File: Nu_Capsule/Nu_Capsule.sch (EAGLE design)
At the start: 20 parts, among them T1 2SC3324, T2 2SC3324

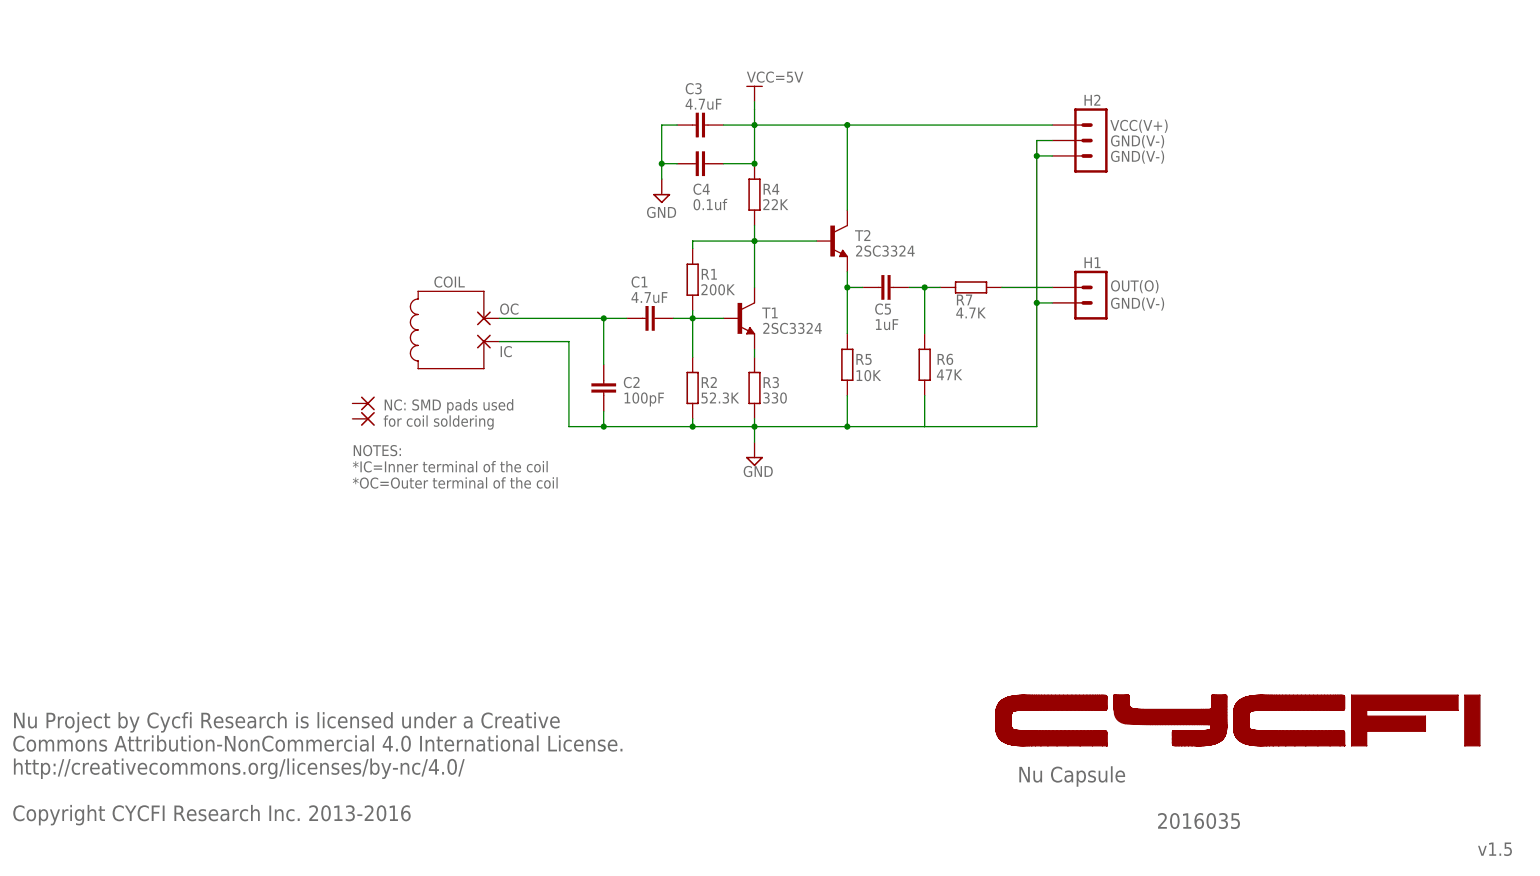
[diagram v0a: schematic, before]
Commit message: Doc updates
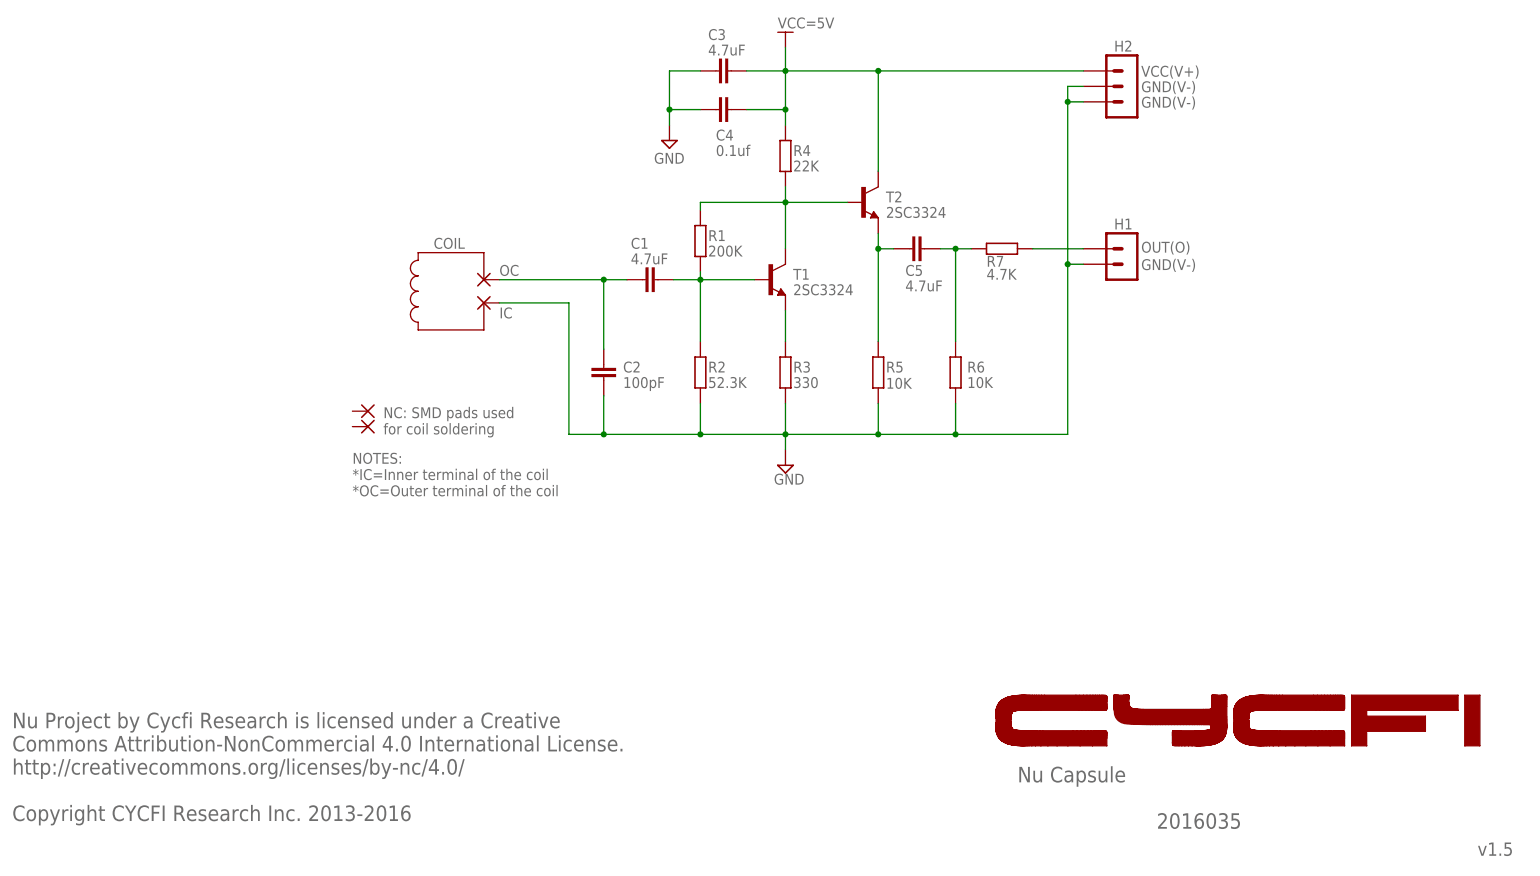
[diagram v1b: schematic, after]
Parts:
- C5: value 1uF -> 4.7uF
- R6: value 47K -> 10K
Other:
- moved on the sheet: C1, C2, C3, C4, C5, H1, H2, R1, R2, R3, R4, R5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

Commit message: updates and minor corrections
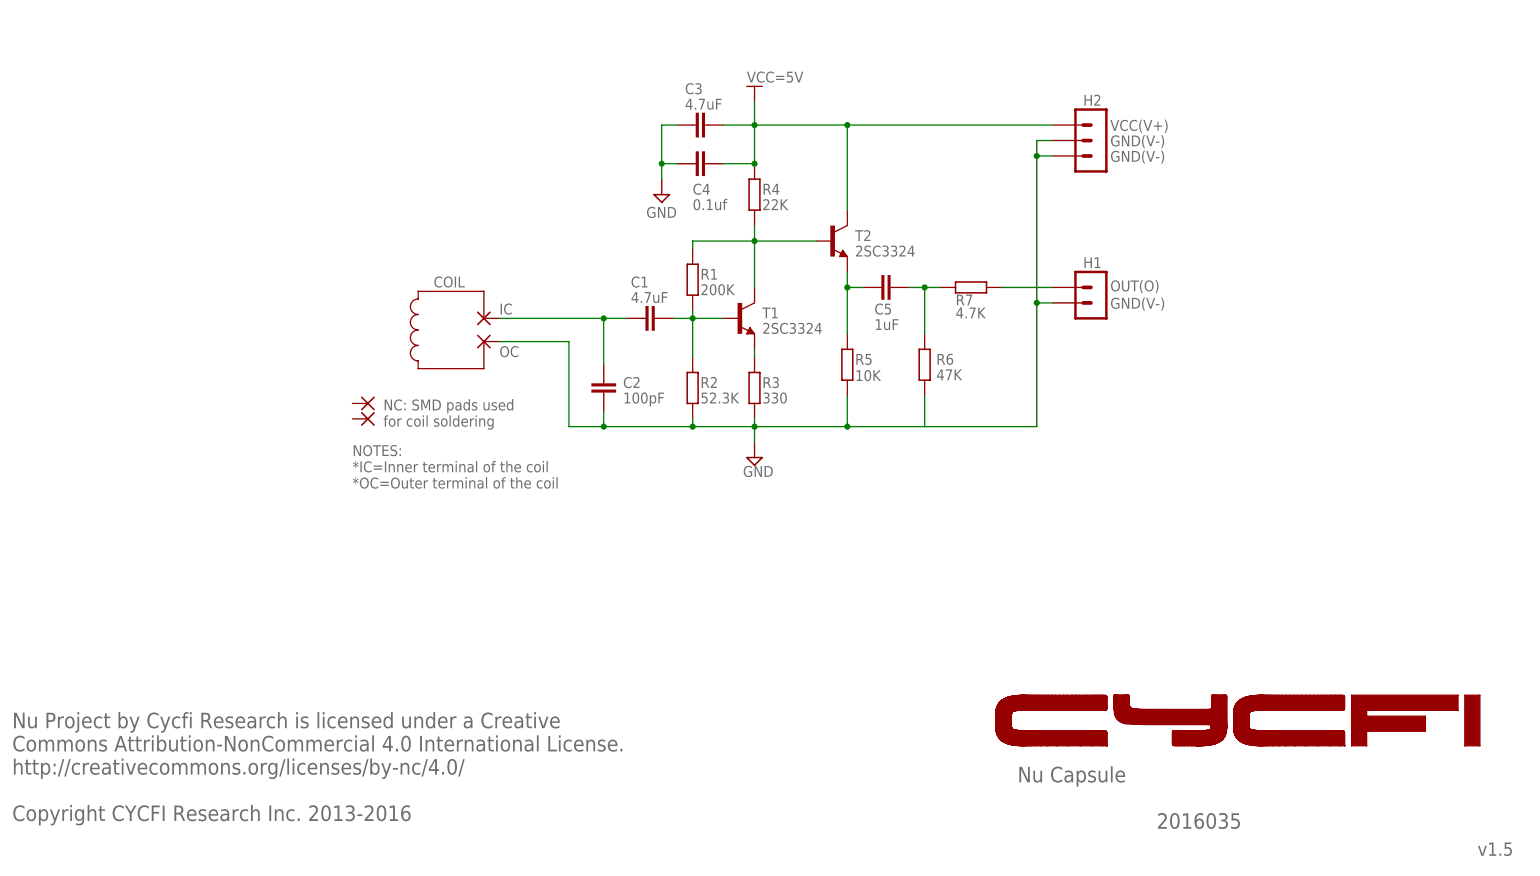
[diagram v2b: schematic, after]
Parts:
- C5: value 4.7uF -> 1uF
- R6: value 10K -> 47K
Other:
- moved on the sheet: C1, C2, C3, C4, C5, H1, H2, R1, R2, R3, R4, R5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

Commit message: more updates; tweaks
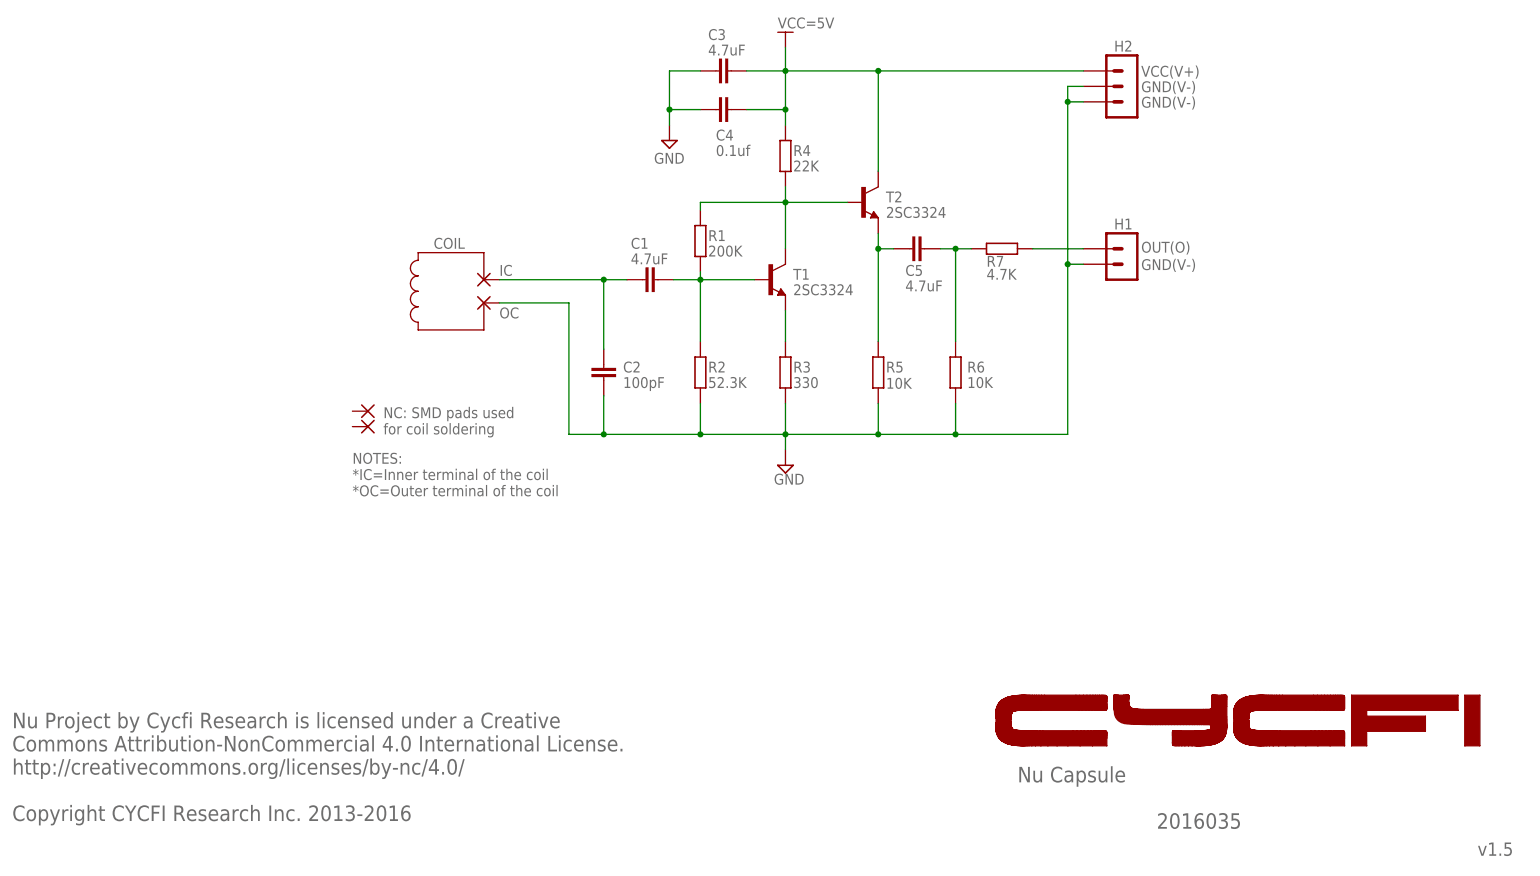
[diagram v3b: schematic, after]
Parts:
- C5: value 1uF -> 4.7uF
- R6: value 47K -> 10K
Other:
- moved on the sheet: C1, C2, C3, C4, C5, H1, H2, R1, R2, R3, R4, R5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

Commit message: Licenses
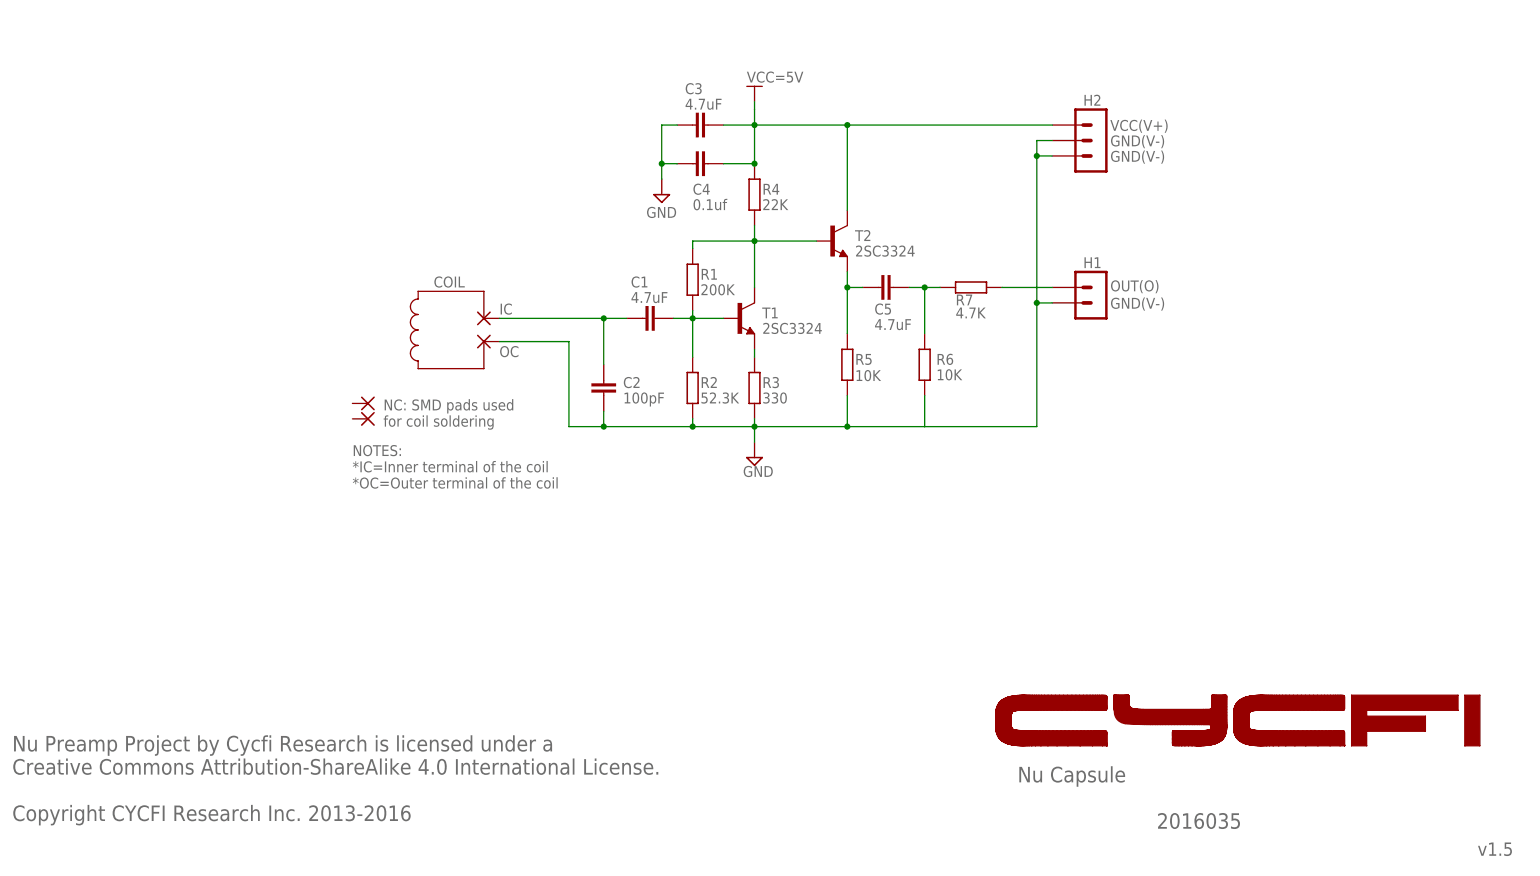
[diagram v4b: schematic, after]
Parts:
- C1, C5: device resistor:C-EUC0805 -> resistor:C-EUC0603
- R2: device resistor:R-EU_R0805 -> resistor:R-EU_R0402
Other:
- note added: "Nu Preamp Project by Cycfi Research is licensed under a Creative Commons Attribution-ShareAlike 4.0 International License. Copyright CYCFI Research Inc. 2013-2016"
- note removed: "Nu Project by Cycfi Research is licensed under a Creative Commons Attribution-NonCommercial 4.0 International License. http://creativecommons.org/licenses/by-nc/4.0/ Copyright CYCFI Research Inc. 2013-2016"
- moved on the sheet: C1, C2, C3, C4, C5, H1, H2, R1, R2, R3, R4, R5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
